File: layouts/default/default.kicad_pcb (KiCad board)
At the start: 2 copper layers, 26 x 27.5 mm, 10 parts

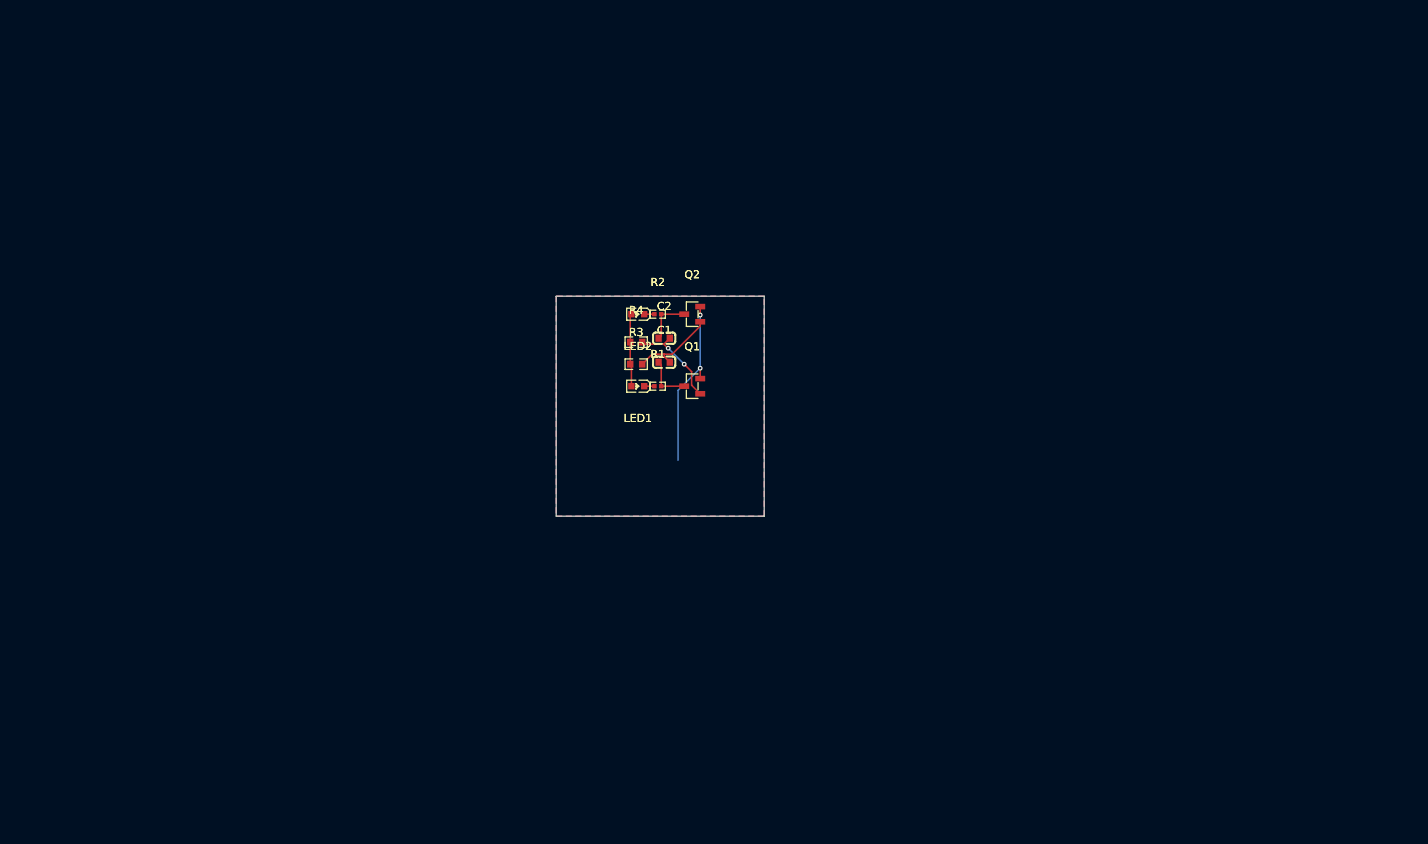
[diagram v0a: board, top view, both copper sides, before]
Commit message: progreesa
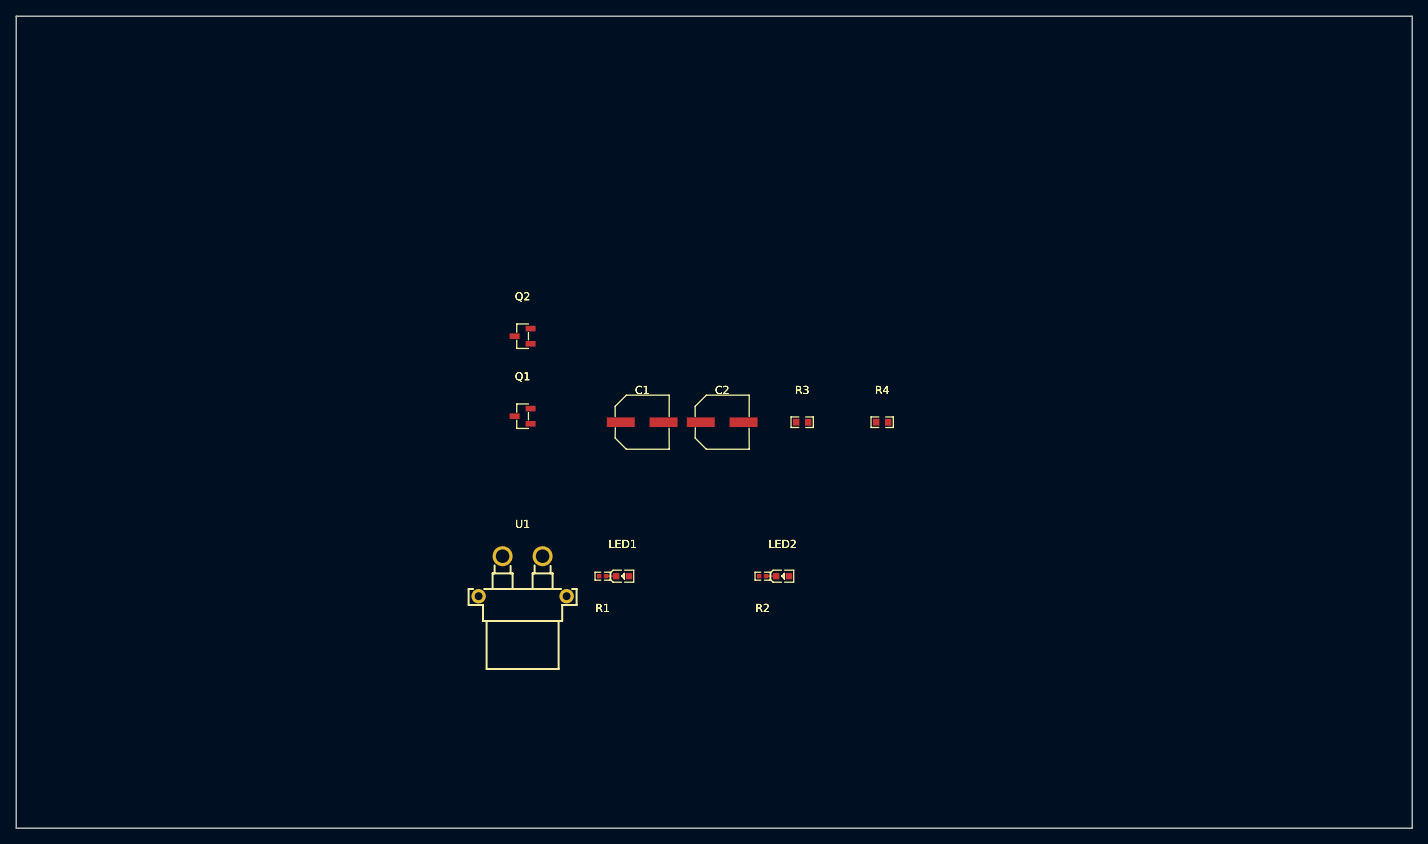
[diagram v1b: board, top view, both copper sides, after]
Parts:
- added U1: , AMASS_XT30PW_F20_G_Y:CONN-TH_XT30PW-F-1, F.Cu at (162.8, 97.0)
- C1, C2: value 10µF ±10% 10V X5R -> (none); footprint Samsung_Electro_Mechanics_CL10A106KP8NNNC:C0603 -> Honor_Elec_RVT1V101M0607:CAP-SMD_BD6.3-L6.6-W6.6-FD
- R4: value 100kΩ ±1% 100mW -> 10kΩ ±1% 100mW; footprint UNI_ROYAL_0603WAF1003T5E:R0603 -> UNI_ROYAL_0603WAF1002T5E:R0603
- moved LED2 37.4 mm to (195.3, 97.0), turned to 0 degrees
- moved R2 35.3 mm to (192.8, 97.0), turned to 180 degrees
- moved R4 32.3 mm to (207.8, 77.8)
- moved R1 24.7 mm to (172.8, 97.0), turned to 180 degrees
- moved LED1 23.8 mm to (175.3, 97.0), turned to 0 degrees
- moved R3 22.0 mm to (197.8, 77.8)
- moved Q1 21.5 mm to (162.8, 77.0)
- moved Q2 21.4 mm to (162.8, 67.0)
- moved C2 12.8 mm to (187.8, 77.8)
- moved C1 7.99 mm to (177.8, 77.8)
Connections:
- net r1.unnamed[1] renamed r1.cathode
- net r2.unnamed[1] renamed r2.cathode
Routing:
- net GND_PAD: track 21.6 -> 0.00 mm, vias 2 -> 0
- net r2.cathode: track 12.0 -> 0.00 mm, vias 2 -> 0
- net r1.cathode: track 11.1 -> 0.00 mm
- net VIN_PAD: track 9.12 -> 0.00 mm
- net led2.low: track 6.01 -> 0.00 mm
- net led1.low: track 6.01 -> 0.00 mm
- removed copper zone on B.Cu, net GND_PAD
- removed copper zone on F.Cu, net GND_PAD
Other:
- board size 26 x 27.5 mm -> 174.5 x 101.5 mm
